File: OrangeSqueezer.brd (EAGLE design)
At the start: 50.5 x 38.1 mm, 31 parts, among them IC1 LM4558N, Q1 2N5457, Q2 2N5457

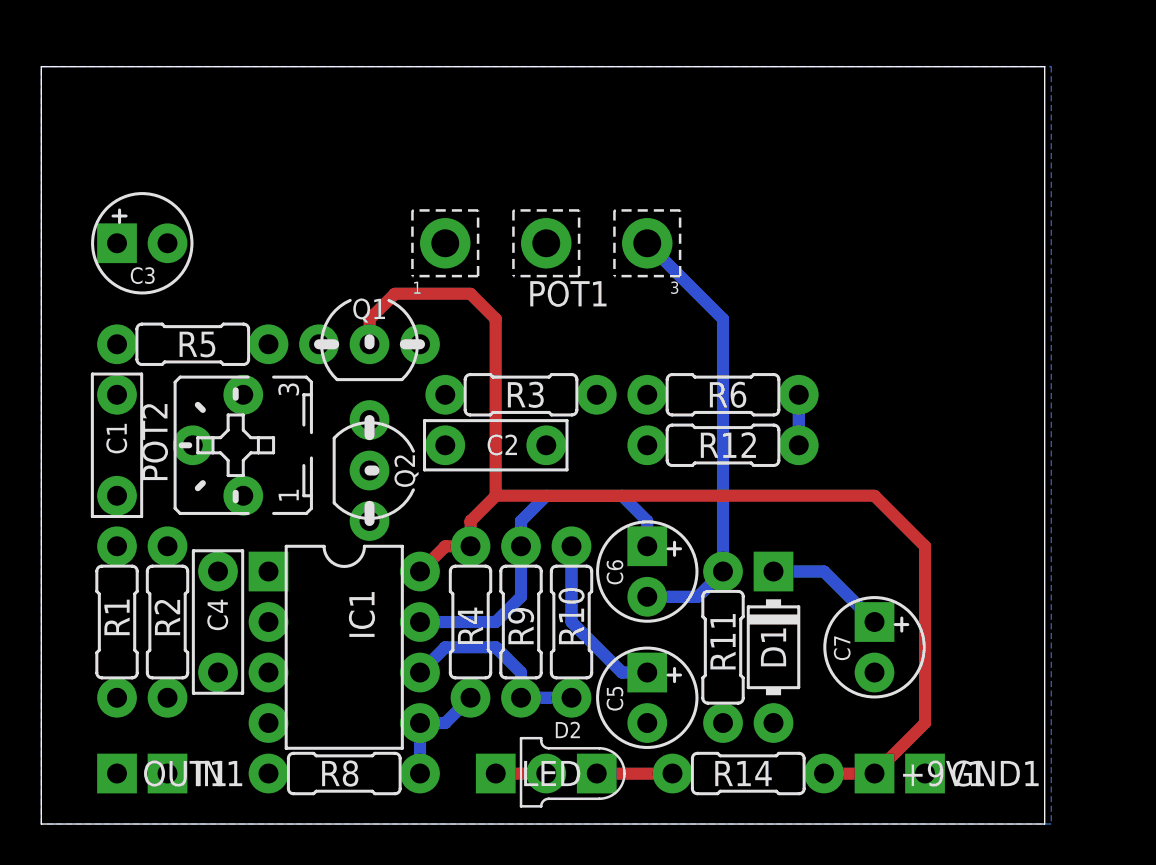
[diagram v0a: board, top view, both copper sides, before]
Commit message: Version 1.0 of Pumpkin Pie sent to Oshpark 12/26/15
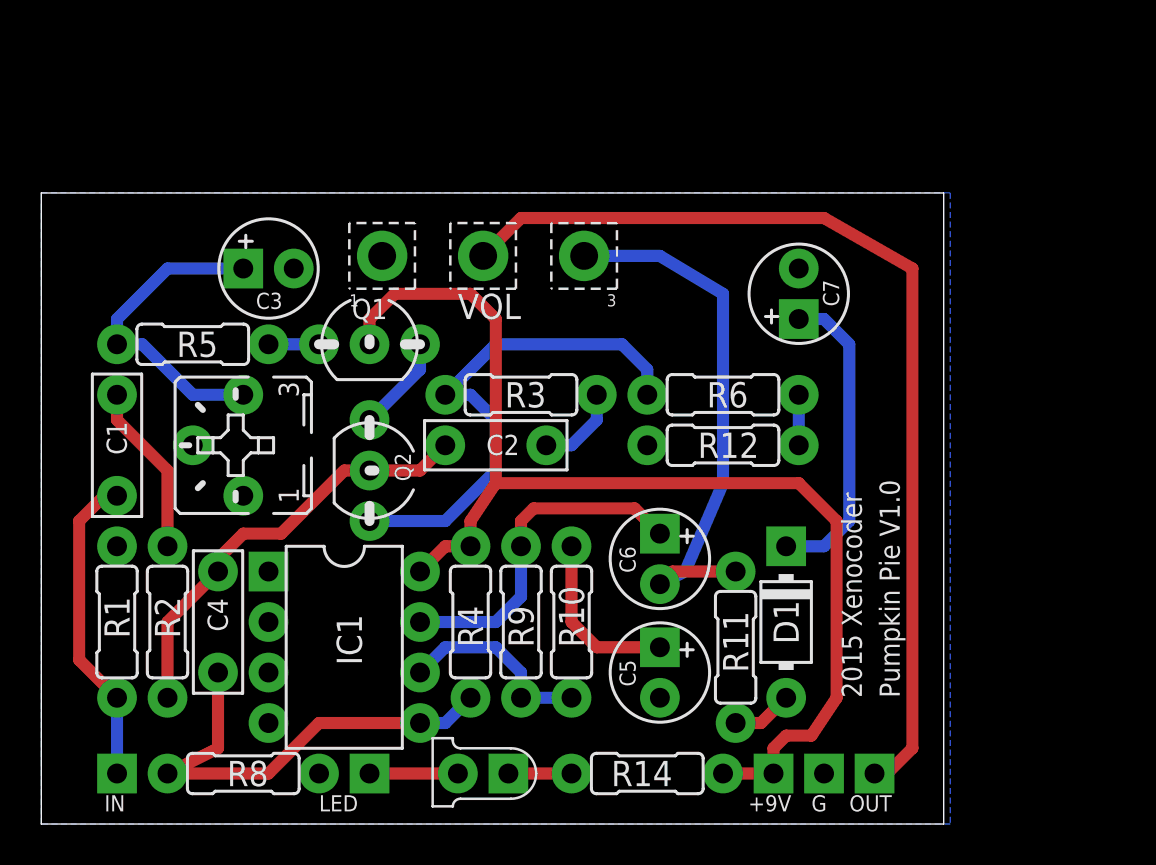
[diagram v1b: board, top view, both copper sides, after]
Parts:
- removed GND1: GND(T), mb_supply:SQUARE
- removed IN1: IN(T), mb_supply:SQUARE
- removed POT1: A10k, mb_pots:16MM_PCB_PADS
- added +9V: +9V(T), mb_supply:SQUARE
- added G: GND(T), mb_supply:SQUARE
- added VOL: A10k, mb_pots:16MM_PCB_PADS
- IN: value OUT(T) -> IN(T)
- OUT: value +9V(T) -> OUT(T)
- moved C7 18.2 mm to (38.1, 26.7), turned to 90 degrees
- moved C3 6.48 mm to (11.4, 27.9)
- moved LED 6.35 mm to (16.5, 2.54)
- moved R14 5.08 mm to (30.5, 2.54)
- moved R8 5.08 mm to (10.2, 2.54), turned to 180 degrees
- moved D2 4.45 mm to (22.2, 2.54)
- moved D1 1.42 mm to (37.5, 10.2)
- moved C5 1.42 mm to (31.1, 7.62)
- moved C6 0.90 mm to (31.1, 13.3)
- moved R11 0.63 mm to (34.9, 8.89)
- renumbered +9V1 to OUT, OUT1 to IN
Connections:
- net +9V: now also +9V.1; no longer OUT.1
- net GND: now also G.1, VOL.1; no longer GND1.1, POT1.1
- net IN: now also IN.1; no longer IN1.1
- net N$12: now also VOL.3; no longer POT1.3
- net OUT: now also OUT.1, VOL.2; no longer IN.1, POT1.2
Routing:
- net OUT: track 0.00 -> 49.6 mm
- net N$7: track 0.00 -> 26.0 mm
- net N$5: track 0.00 -> 21.8 mm
- net N$9: track 5.61 -> 23.5 mm
- net N$8: track 0.00 -> 16.1 mm
- net IN: track 0.00 -> 15.9 mm
- net N$14: track 6.13 -> 15.7 mm
- net N$1: track 0.00 -> 8.67 mm
- net N$12: track 22.4 -> 27.4 mm
- net N$3: track 0.00 -> 4.86 mm
- net N$6: track 0.00 -> 4.34 mm
- net N$13: track 0.00 -> 3.07 mm
- net +9V: track 61.4 -> 58.6 mm
- net N$2: track 0.00 -> 2.54 mm
- net N$16: track 2.54 -> 4.44 mm
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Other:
- board size 50.5 x 38.1 mm -> 45.4 x 31.7 mm
- board text added: "2015 Xenocoder"
- board text added: "Pumpkin Pie V1.0"

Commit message: First commit for The Thing tremolo
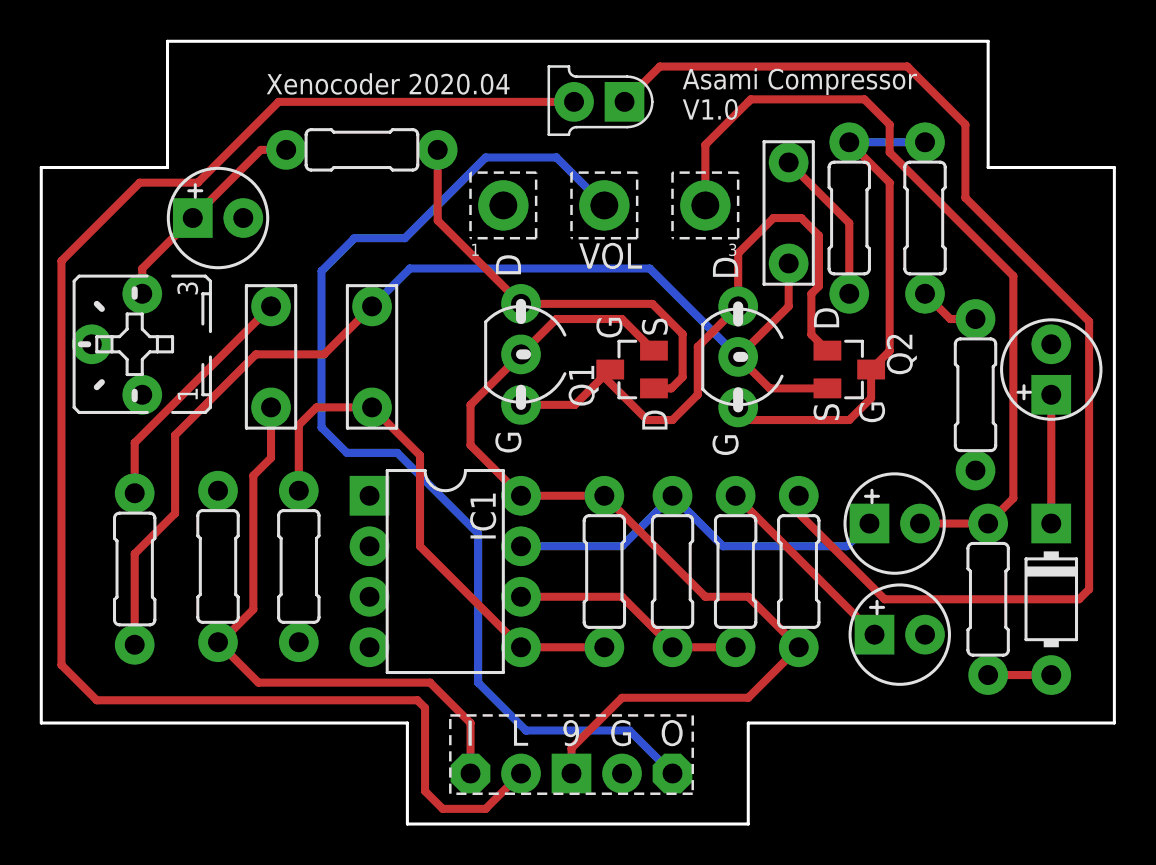
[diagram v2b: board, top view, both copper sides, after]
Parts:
- removed +9V: +9V(T), mb_supply:SQUARE
- removed G: GND(T), mb_supply:SQUARE
- removed IN: IN(T), mb_supply:SQUARE
- removed LED: LED, mb_supply:SQUARE
- removed OUT: OUT(T), mb_supply:SQUARE
- added Q3, Q4: 2N5457, xc_library:TO92-
- added U$1: BOARDLINK, xc_library:BOARDLINK
- C1, C4: value 0.047uF -> 47nF
- C2: value 0.0022uF -> 2n2
- Q1, Q2: value 2N5457 -> MMBF5457; device mb_trans:TO92- -> xc_library:SOT23
- moved D2 34.3 mm to (28.1, 36.3)
- moved Q2 24.7 mm to (40.6, 22.9)
- moved C2 18.8 mm to (37.6, 30.7), turned to 270 degrees
- moved R3 18.8 mm to (40.6, 30.5), turned to 90 degrees
- moved C4 15.4 mm to (16.6, 23.5)
- moved R6 13.5 mm to (44.5, 30.5), turned to 90 degrees
- moved D1 13.4 mm to (50.8, 11.3)
- moved Q1 13.3 mm to (29.7, 22.9), turned to 90 degrees
- moved C7 13.3 mm to (50.8, 22.9)
- moved R5 13.0 mm to (16.1, 33.9)
- moved R12 13.0 mm to (47.0, 21.6), turned to 90 degrees
- moved R11 12.9 mm to (47.6, 11.3)
- moved R14 12.7 mm to (38.1, 12.7), turned to 90 degrees
- moved C5 12.2 mm to (43.2, 9.53), turned to 0 degrees
- moved C6 11.9 mm to (42.9, 15.1), turned to 0 degrees
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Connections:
- removed net IN: C1.2, IN.1, R1.2
- removed net OUT: OUT.1, VOL.2
- new net N$10: U$1.5, VOL.2
- new net N$20: C1.2, R1.2, U$1.1
- net +9V: now also Q3.2, U$1.3; no longer +9V.1
- net GND: now also U$1.4; no longer G.1
- net N$16: now also U$1.2; no longer LED.1
- net N$2: now also Q1.1, Q3.3; no longer Q1.3
- net N$3: now also Q1.3, Q2.1, Q3.1, Q4.3; no longer Q1.1, Q2.3
- net N$5: now also Q4.2
- net N$7: now also Q2.3, Q4.1; no longer Q2.1
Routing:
- net N$16: track 4.44 -> 78.7 mm
- net N$15: track 3.18 -> 62.5 mm
- net N$10: track 0.00 -> 54.7 mm
- net OUT: track 49.6 -> 0.00 mm
- net N$5: track 21.8 -> 55.9 mm
- net N$20: track 0.00 -> 29.9 mm
- net N$3: track 4.86 -> 30.8 mm
- net N$2: track 2.54 -> 22.1 mm
- net IN: track 15.9 -> 0.00 mm
- net N$12: track 27.4 -> 40.4 mm
- net +9V: track 58.6 -> 49.2 mm
- net N$14: track 15.7 -> 6.48 mm
- net N$8: track 16.1 -> 11.0 mm
- net N$1: track 8.67 -> 12.2 mm
- net N$6: track 4.34 -> 7.87 mm
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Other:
- board size 45.4 x 31.7 mm -> 54 x 39.4 mm
- board text added: "Asami Compressor V1.0"
- board text added: "Xenocoder 2020.04"
- board text removed: "2015 Xenocoder"
- board text removed: "Pumpkin Pie V1.0"
